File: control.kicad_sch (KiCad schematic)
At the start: 40 parts, among them J4 Conn_01x05_Pin, J5 Conn_01x03_Pin, J6 Conn_01x03_Pin, Q2 AO3400, Q3 DTC143Z, Q4 DMG1012T, SW2 SW_Push, SW3 SW_SPDT, U6 STM32G031G8Ux

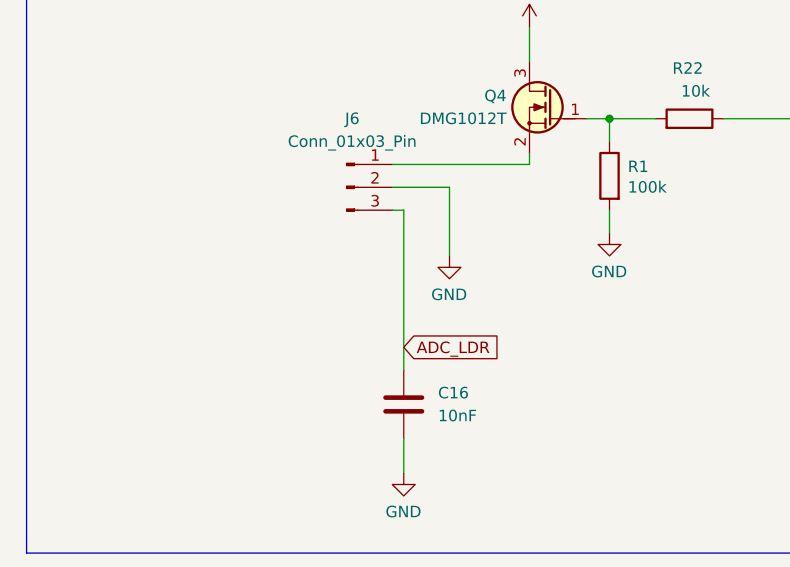
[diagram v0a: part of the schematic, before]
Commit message: Finished v3
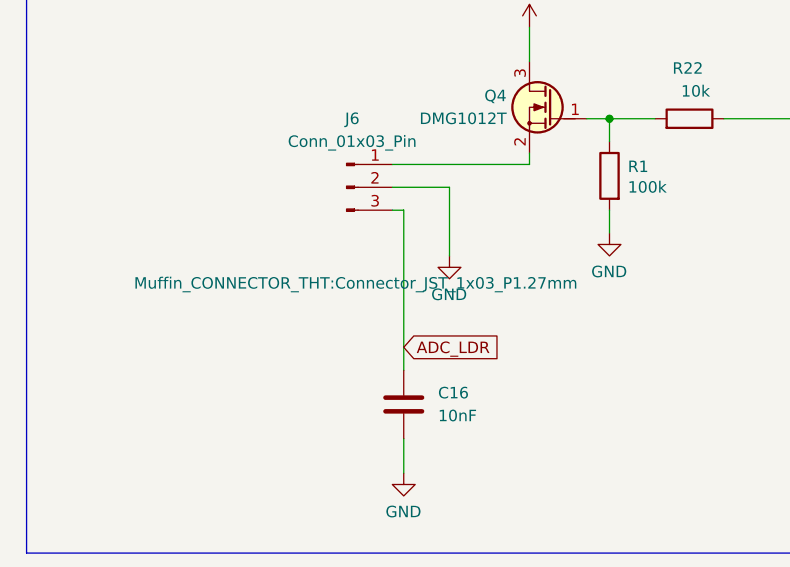
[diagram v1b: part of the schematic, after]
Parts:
- J6: footprint conn:PinHeader_1x03_P1.27mm_Vertical -> Muffin_CONNECTOR_THT:Connector_JST_1x03_P1.27mm
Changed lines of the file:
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@@
 		(on_board yes)
 		(dnp no)
-		(fields_autoplaced yes)
 		(property "Reference" "J6"
 			(at 56.515 144.78 0)
@@
 			)
 		)
-		(property "Footprint" "conn:PinHeader_1x03_P1.27mm_Vertical"
-			(at 55.88 152.4 0)
+		(property "Footprint" "Muffin_CONNECTOR_THT:Connector_JST_1x03_P1.27mm"
+			(at 56.896 163.068 0)
 			(effects
 				(font
 					(size 1.27 1.27)
 				)
-				(hide yes)
 			)
 		)
